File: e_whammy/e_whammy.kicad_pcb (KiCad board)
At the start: 4 copper layers, 30 x 12 mm, 18 parts, among them J1 I/O connector, U1 HT7550-1, U2 DRV5056, U3 TLV6001UIDBVR

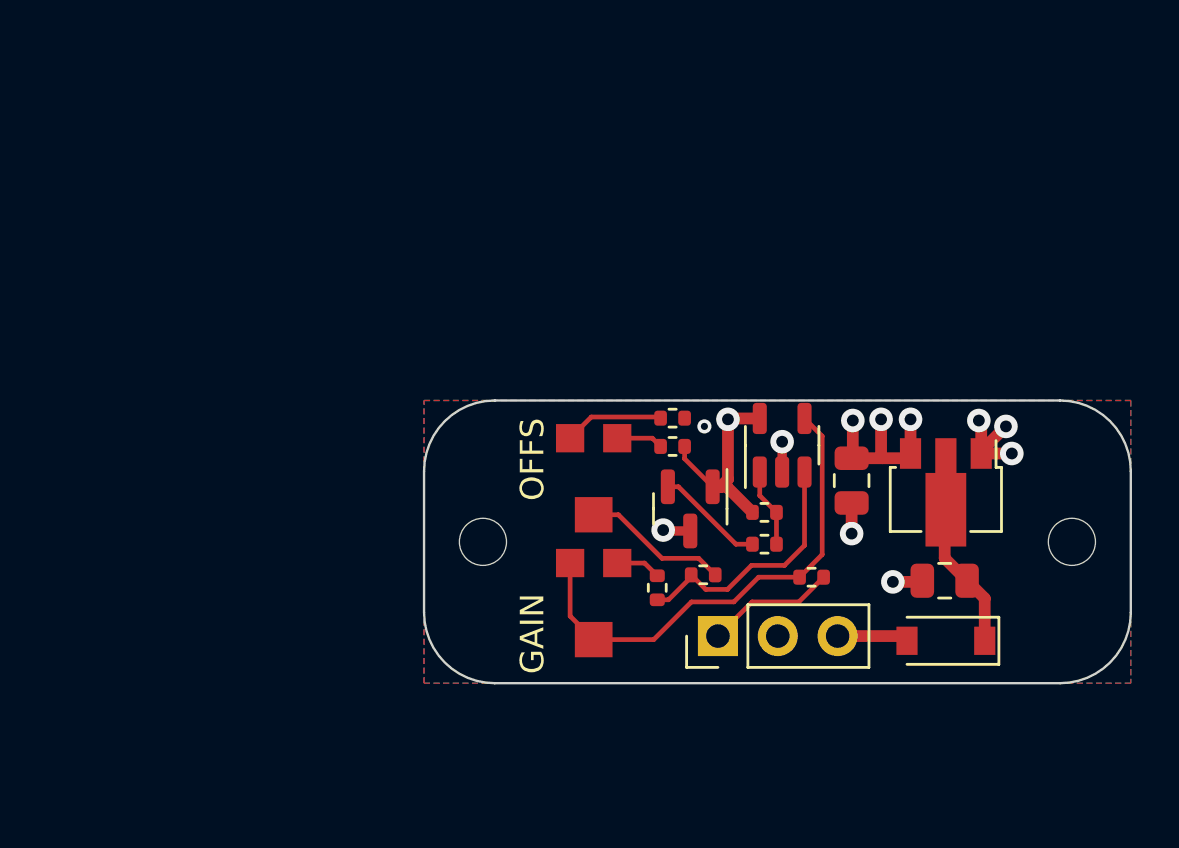
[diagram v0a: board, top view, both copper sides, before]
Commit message: New uni-mount version
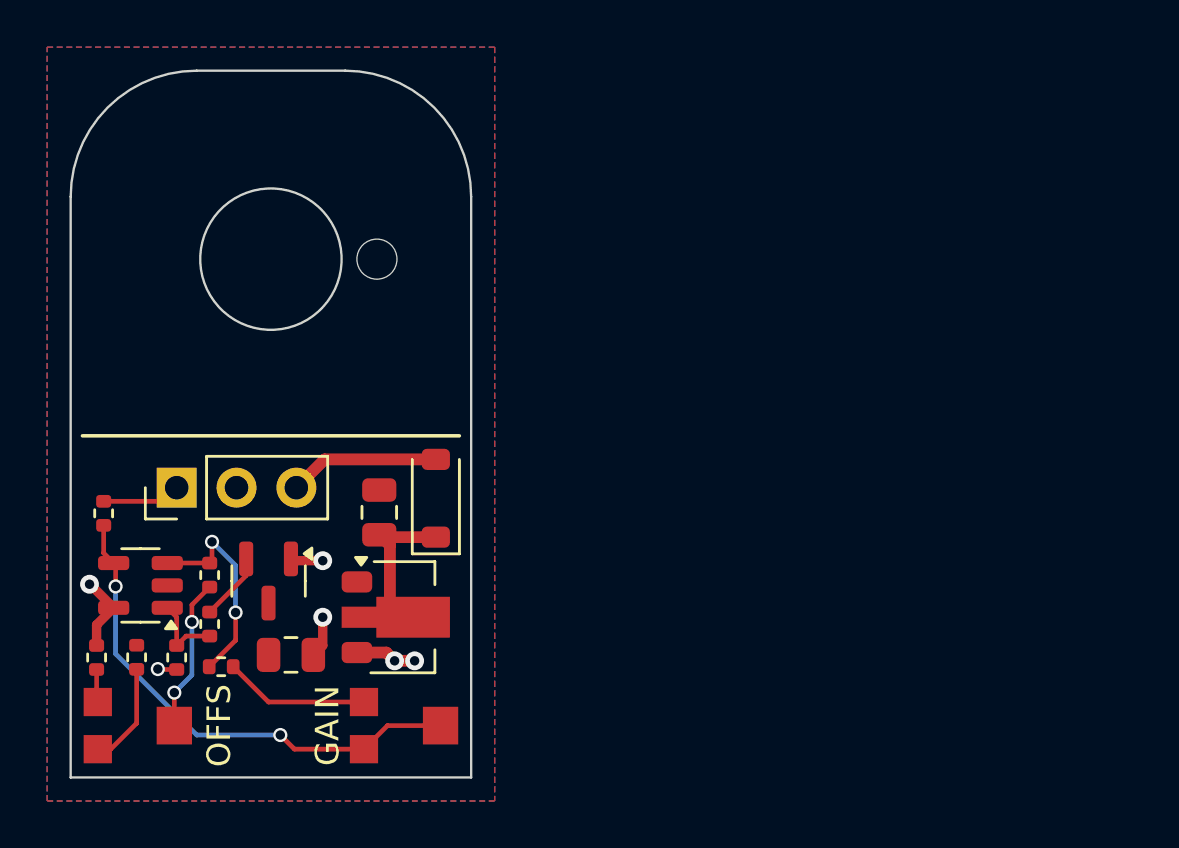
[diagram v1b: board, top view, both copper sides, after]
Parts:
- removed the REF** at (152.5, 110.0)
- removed the REF** at (127.5, 110.0)
- added REF**: hole_1.7mm, cycfi_library:hole_1.7mm, F.Cu at (123.0, 98.0)
- moved R7 30.2 mm to (111.4, 108.8), turned to 90 degrees
- moved U3 27.9 mm to (113.0, 111.8), turned to 180 degrees
- moved R2 26.0 mm to (111.1, 114.9), turned to 90 degrees
- moved R5 25.7 mm to (114.5, 114.9), turned to -90 degrees
- moved C2 24.9 mm to (119.3, 114.8), turned to 180 degrees
- moved R1 24.9 mm to (112.8, 114.9), turned to -90 degrees
- moved C1 24.2 mm to (123.1, 108.8), turned to 90 degrees
- moved J1 23.8 mm to (114.5, 107.7)
- moved R3 23.8 mm to (115.9, 113.5), turned to -90 degrees
- moved U1 23.7 mm to (124.1, 113.2), turned to 0 degrees
- moved D1 22.5 mm to (125.5, 108.2), turned to 90 degrees
- moved RV1 21.9 mm to (113.0, 117.8), turned to -90 degrees
- moved R4 21.0 mm to (115.9, 111.4), turned to 90 degrees
- moved R6 18.8 mm to (116.4, 115.3), turned to 0 degrees
- moved U2 18.2 mm to (118.4, 111.7)
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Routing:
- net GND: track 9.35 -> 0.00 mm, vias 8 -> 0
- net 5v: track 16.4 -> 9.59 mm, vias 4 -> 6
- net Net-(R6-Pad2): track 1.92 -> 6.17 mm
- net V+: track 3.03 -> 6.42 mm
- net OUT: track 5.52 -> 3.34 mm
- net Net-(U3--): track 10.9 -> 8.92 mm, vias 0 -> 2
- net Net-(D1-K): track 8.59 -> 6.79 mm
- net Net-(U2-OUT): track 4.60 -> 2.90 mm
- net Net-(R7-Pad1): track 20.9 -> 21.5 mm, vias 0 -> 2
- net Net-(R2-Pad1): track 1.98 -> 1.40 mm
- net Net-(R4-Pad1): track 6.22 -> 6.50 mm, vias 0 -> 2
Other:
- board size 30 x 12 mm -> 17 x 30 mm
